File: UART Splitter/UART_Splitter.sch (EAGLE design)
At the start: 31 parts, among them IC1 ATTINY10, Q1 12mhz, U1 74HC4052

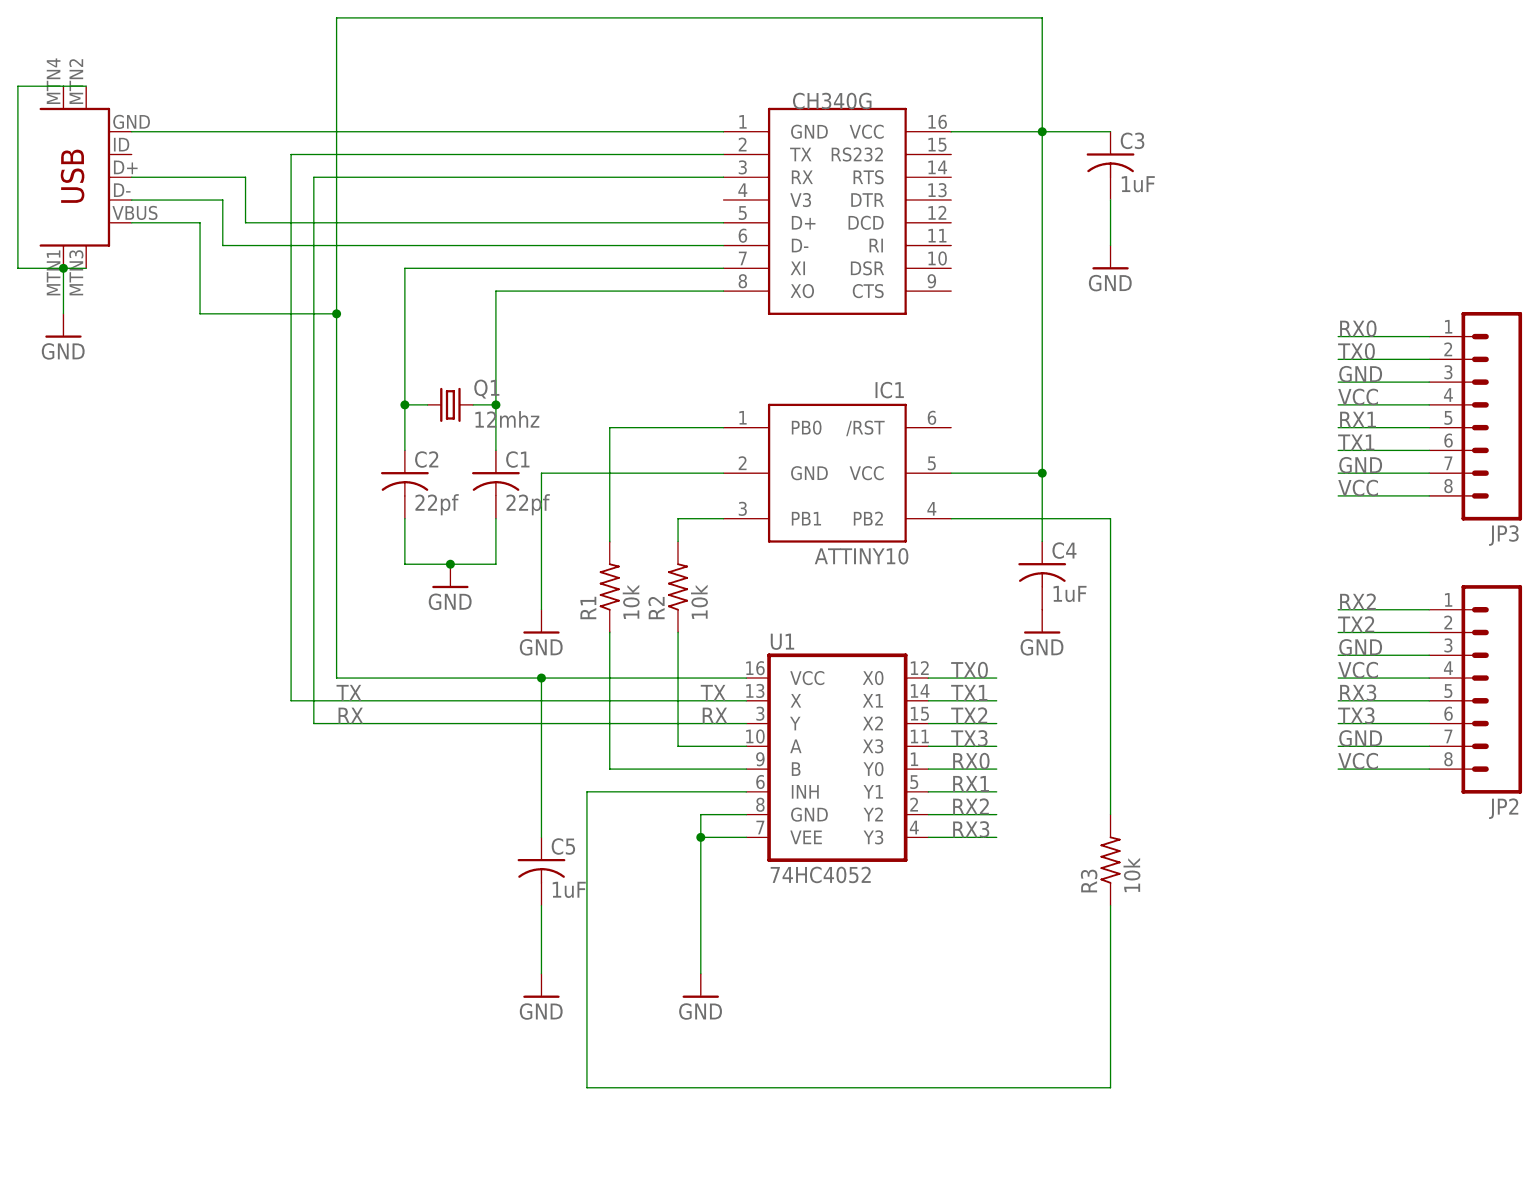
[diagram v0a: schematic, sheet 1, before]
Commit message: UART Splitter
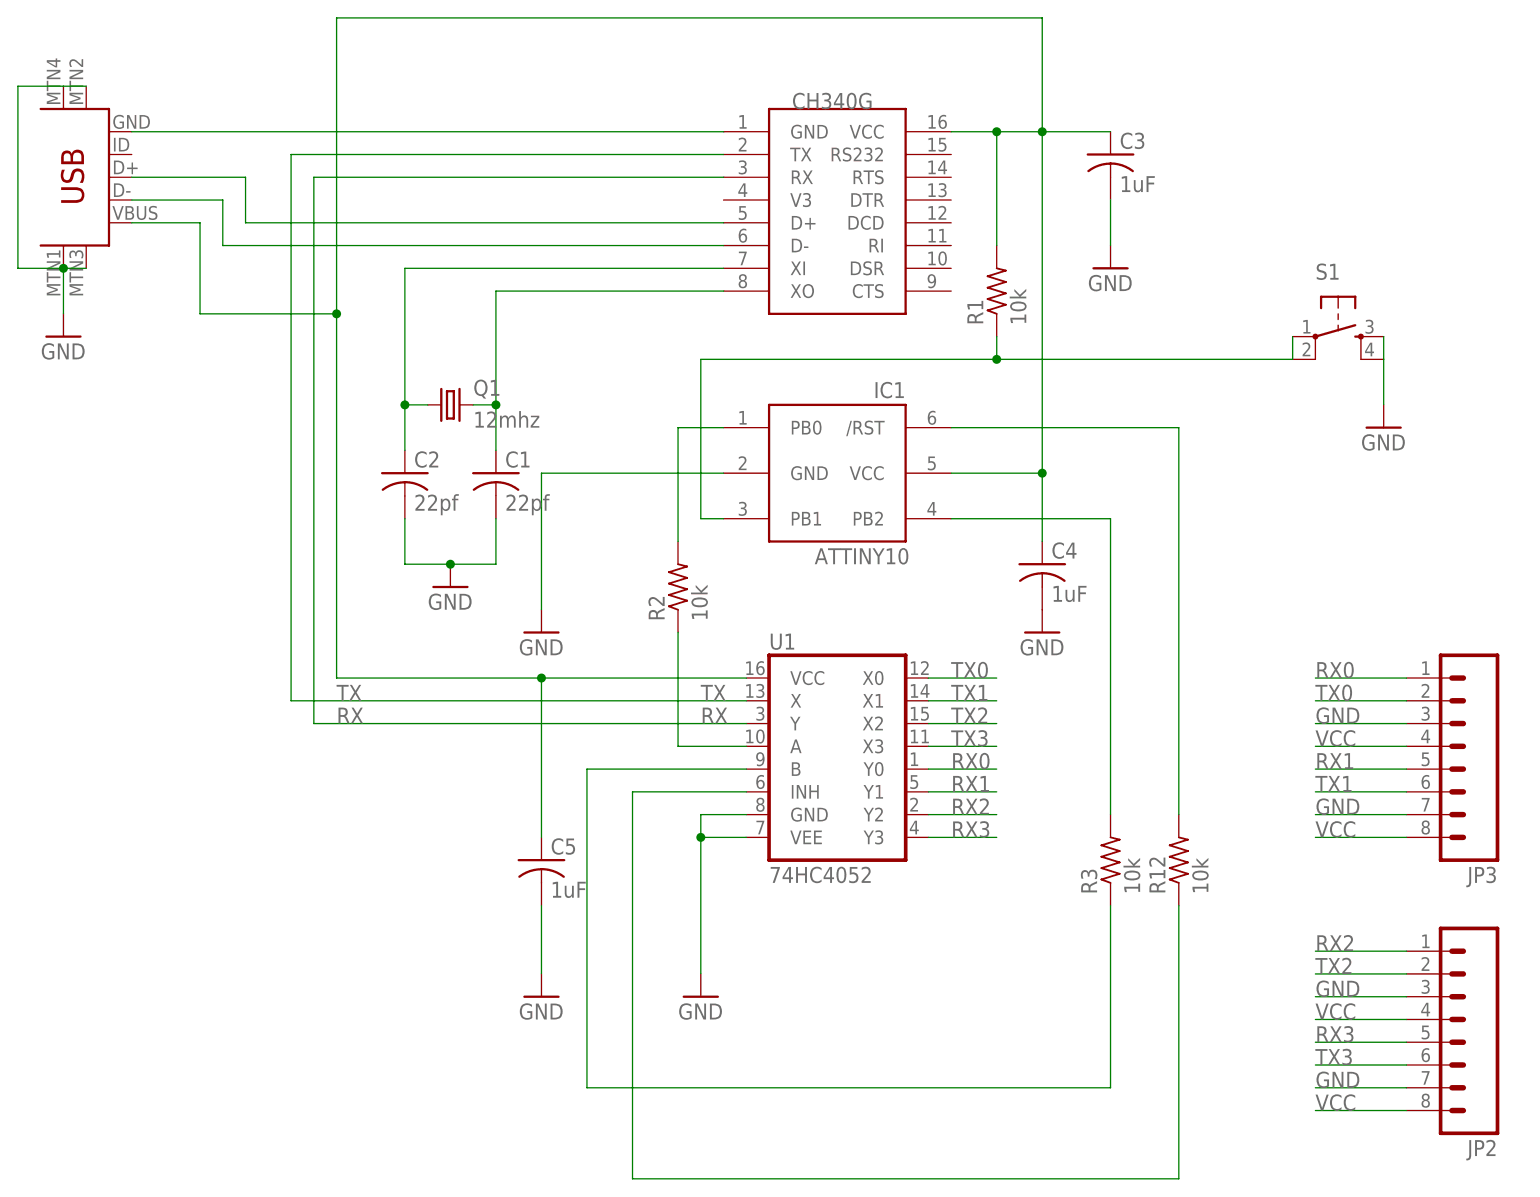
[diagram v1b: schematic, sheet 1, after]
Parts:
- added R12: 10k, resistor:R-US_R0402
- added S1: (no value), SparkFun-Electromechanical:TAC_SWITCHSMD
- C1, C2, C3, C4, C5: device resistor:C-USC0805K -> resistor:C-USC0402K
- R1, R10, R11, R2, R3, R4, R5, R6, R7, R8, R9: device resistor:R-US_R0805W -> resistor:R-US_R0402
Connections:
- new net N$13: R12.1, U1.INH
- net GND: now also S1.3, S1.4
- net N$2: now also R1.2
- net N$6: no longer R1.1
- net N$7: now also IC1.PB1, R1.1, S1.1, S1.2; no longer U1.INH
- net N$8: now also IC1./RST, R12.2; no longer IC1.PB0, R1.2
- net N$9: now also IC1.PB0; no longer IC1.PB1
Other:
- moved on the sheet: JP2, JP3, R1
